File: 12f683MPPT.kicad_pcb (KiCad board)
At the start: 2 copper layers, 98.3 x 72.6 mm, 54 parts, among them J1 Conn_01x01_Male, J2 Conn_01x01_Male, J3 Conn_01x01_Male, J4 Conn_01x01_Male, Q1 BUK9511-55A127, Q2 BUK9511-55A127, Q3 2N2222A, Q4 2N2222A, Q5 2N2907A, SW1 SW_Push, U1 LM7805_TO220, U2 PIC12F683-IP, U3 LM358

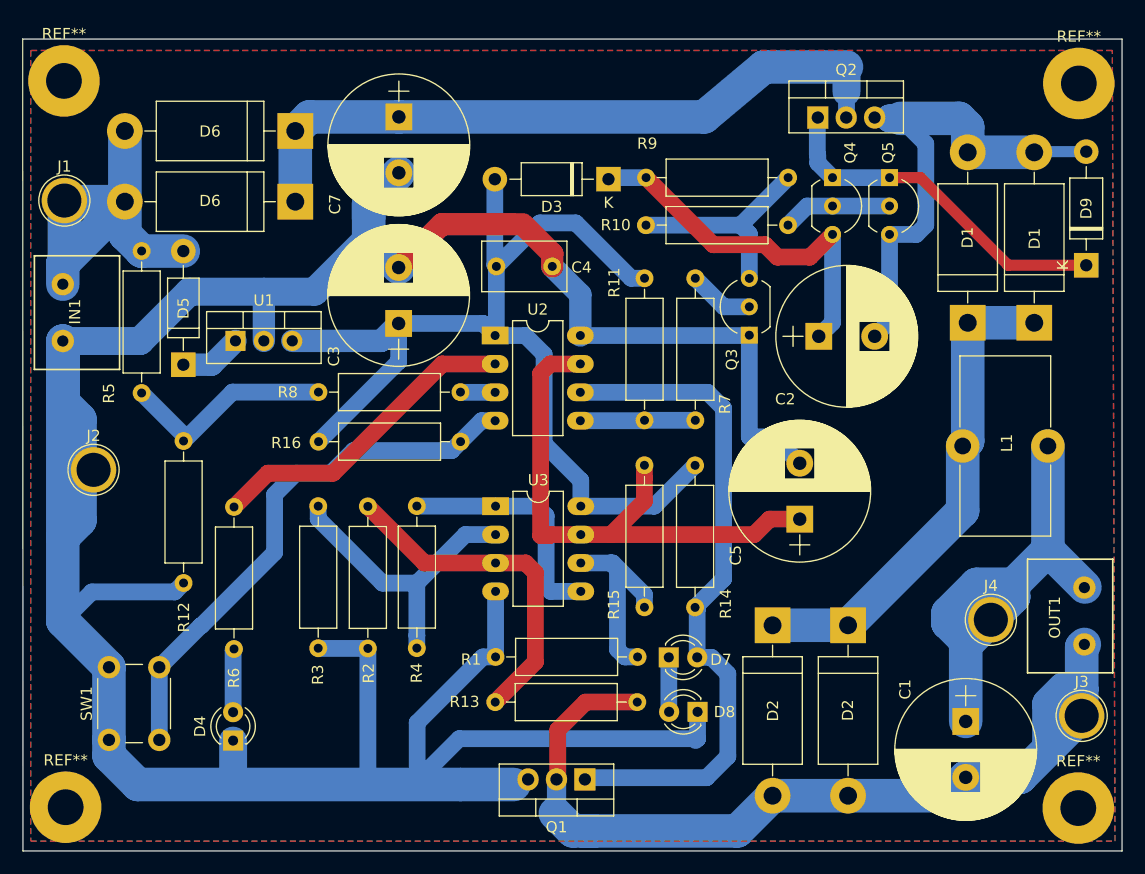
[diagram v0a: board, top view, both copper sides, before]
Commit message: Update circuit.
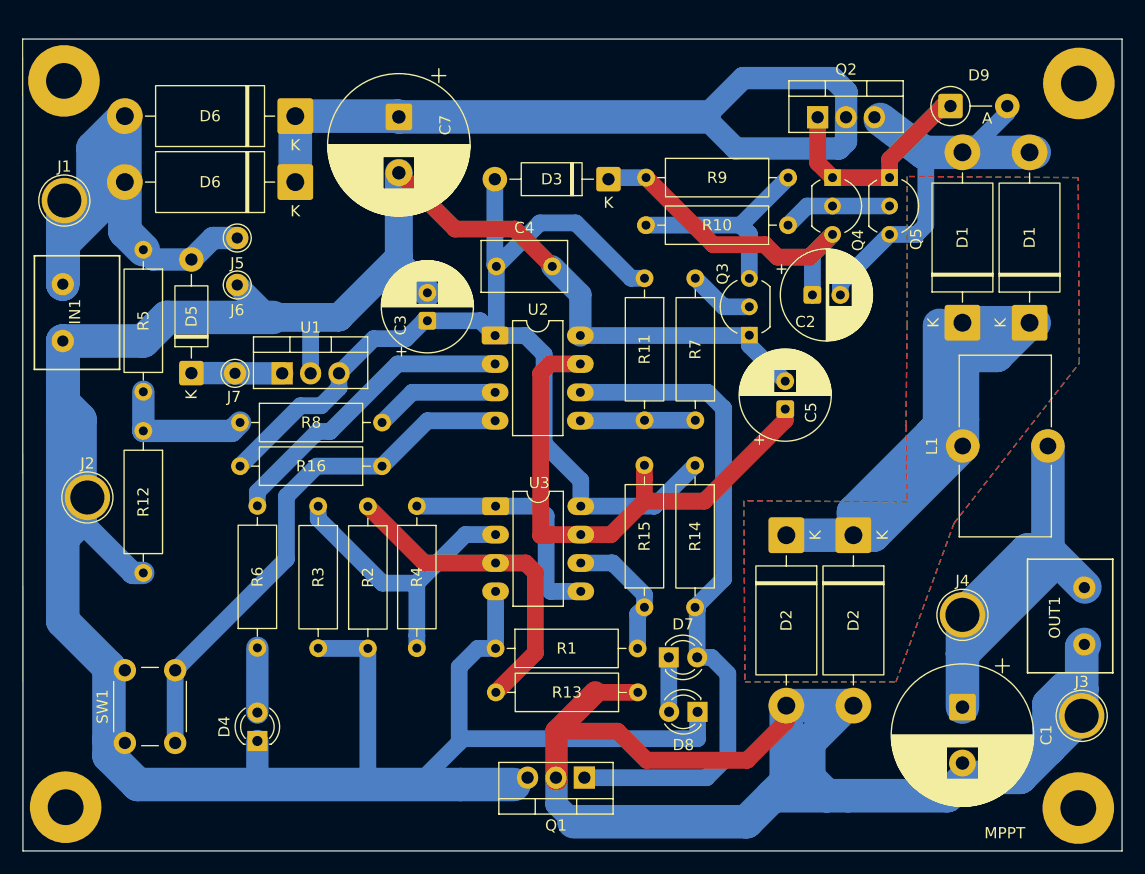
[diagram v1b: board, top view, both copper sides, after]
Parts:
- added J5: Vin, Connector_Pin:Pin_D1.0mm_L10.0mm, F.Cu at (55.4, 44.3)
- added J6: GND, Connector_Pin:Pin_D1.0mm_L10.0mm, F.Cu at (55.4, 48.5)
- added J7: 12V, Connector_Pin:Pin_D1.0mm_L10.0mm, F.Cu at (55.2, 56.4)
- C1, C7: footprint Capacitors_THT:CP_Radial_D12.5mm_P5.00mm -> Capacitor_THT:CP_Radial_D12.5mm_P5.00mm
- C2, C3, C5: footprint Capacitors_THT:CP_Radial_D12.5mm_P5.00mm -> Capacitor_THT:CP_Radial_D8.0mm_P2.50mm
- C4: footprint Capacitors_THT:C_Disc_D7.5mm_W4.4mm_P5.00mm -> Capacitor_THT:C_Disc_D7.5mm_W4.4mm_P5.00mm
- D1 (x2), D2 (x2), D6 (x2): footprint Diodes_THT:D_DO-201AD_P15.24mm_Horizontal -> Diode_THT:D_DO-201AD_P15.24mm_Horizontal
- D4, D7, D8: footprint LEDs:LED_D3.0mm -> LED_THT:LED_D3.0mm
- D5: footprint Diodes_THT:D_DO-41_SOD81_P10.16mm_Horizontal -> Diode_THT:D_DO-41_SOD81_P10.16mm_Horizontal
- D9: footprint Diode_THT:D_DO-41_SOD81_P10.16mm_Horizontal -> Diode_THT:D_DO-41_SOD81_P5.08mm_Vertical_AnodeUp
- L1: footprint Inductors_THT:L_Toroid_Vertical_L16.0mm_W8.0mm_P7.62mm -> Inductor_THT:L_Toroid_Vertical_L16.0mm_W8.0mm_P7.62mm
- Q3, Q4, Q5: footprint TO_SOT_Packages_THT:TO-92_Inline_Wide -> Package_TO_SOT_THT:TO-92_Inline_Wide
- R1, R10, R11, R12, R13, R14, R15, R16, R2, R3, R4, R5, R6, R7, R8, R9: footprint Resistors_THT:R_Axial_DIN0309_L9.0mm_D3.2mm_P12.70mm_Horizontal -> Resistor_THT:R_Axial_DIN0309_L9.0mm_D3.2mm_P12.70mm_Horizontal
- U1: footprint TO_SOT_Packages_THT:TO-220-3_Vertical -> Package_TO_SOT_THT:TO-220-3_Vertical
- U2, U3: footprint Housings_DIP:DIP-8_W7.62mm_LongPads -> Package_DIP:DIP-8_W7.62mm_LongPads
- moved D9 18.7 mm to (119.2, 32.5), turned to 0 degrees
- moved C5 9.93 mm to (104.4, 59.6)
- moved D2 8.15 mm to (104.5, 70.9)
- moved D2 8.07 mm to (110.5, 70.9)
- moved R8 7.52 mm to (55.6, 60.8)
- moved R16 7.35 mm to (68.3, 64.7)
- moved U1 5.09 mm to (59.4, 56.4)
- moved C2 3.74 mm to (106.8, 49.4)
- moved R12 3.71 mm to (47.0, 61.5)
- moved C3 2.58 mm to (72.4, 51.7)
- moved J4 2.58 mm to (120.2, 78.0)
- moved J2 2.53 mm to (42.0, 67.5)
- moved D4 2.17 mm to (57.2, 89.3)
- moved R6 2.09 mm to (57.2, 81.0)
- moved D6 1.75 mm to (60.6, 39.3)
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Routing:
- net PRI_LO: track 98.8 -> 130.9 mm
- net Net-(D1-K): track 44.6 -> 65.2 mm
- net Net-(D6-K): track 62.4 -> 75.8 mm
- net +24V: track 35.9 -> 48.5 mm
- net Net-(D9-K): track 31.8 -> 20.1 mm
- net GNDPWR: track 319.0 -> 310.1 mm
- net /PV-Voltage: track 3.11 -> 11.2 mm
- net Net-(R12-Pad1): track 19.7 -> 12.5 mm
- net Net-(D1-A): track 45.4 -> 38.5 mm
- net Net-(U3B--): track 18.0 -> 11.9 mm
- net PRI_HI: track 49.6 -> 44.7 mm
- net Net-(D3-A): track 97.2 -> 92.4 mm
- net /BootStrap: track 33.6 -> 30.2 mm
- net Net-(D5-K): track 5.54 -> 8.13 mm
- net Net-(U2-GP5): track 28.6 -> 27.2 mm
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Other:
- board text added: "MPPT"
